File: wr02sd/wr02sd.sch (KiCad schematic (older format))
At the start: 9 parts

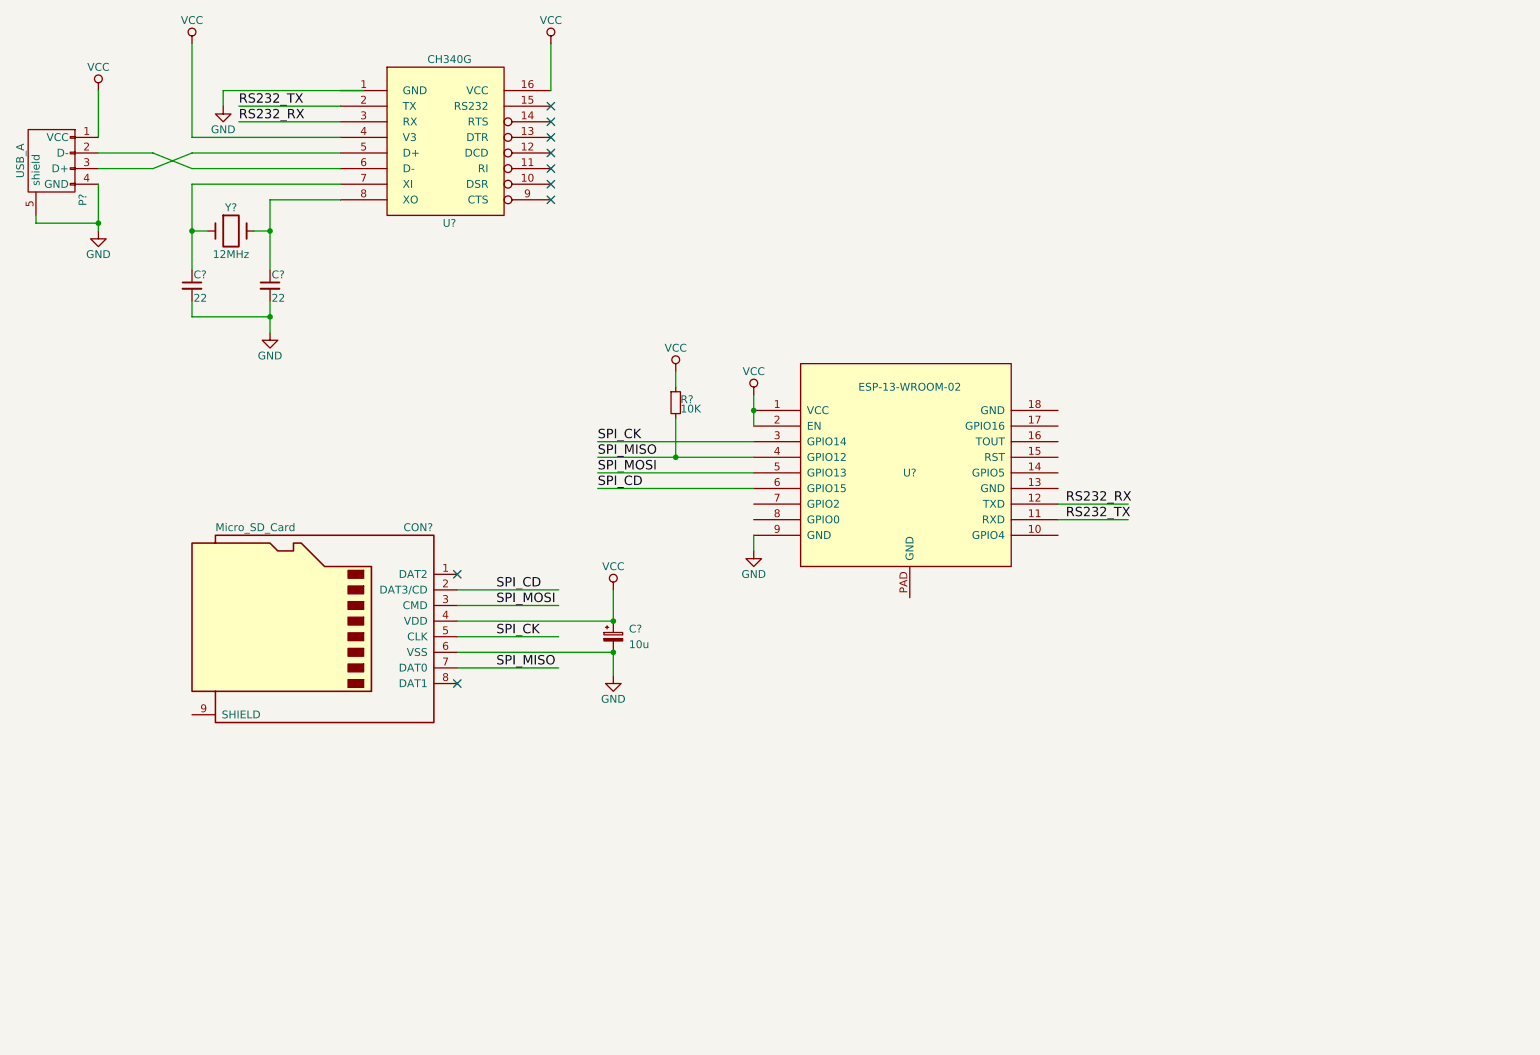
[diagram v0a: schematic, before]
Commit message: PCB Artworking is progressing.
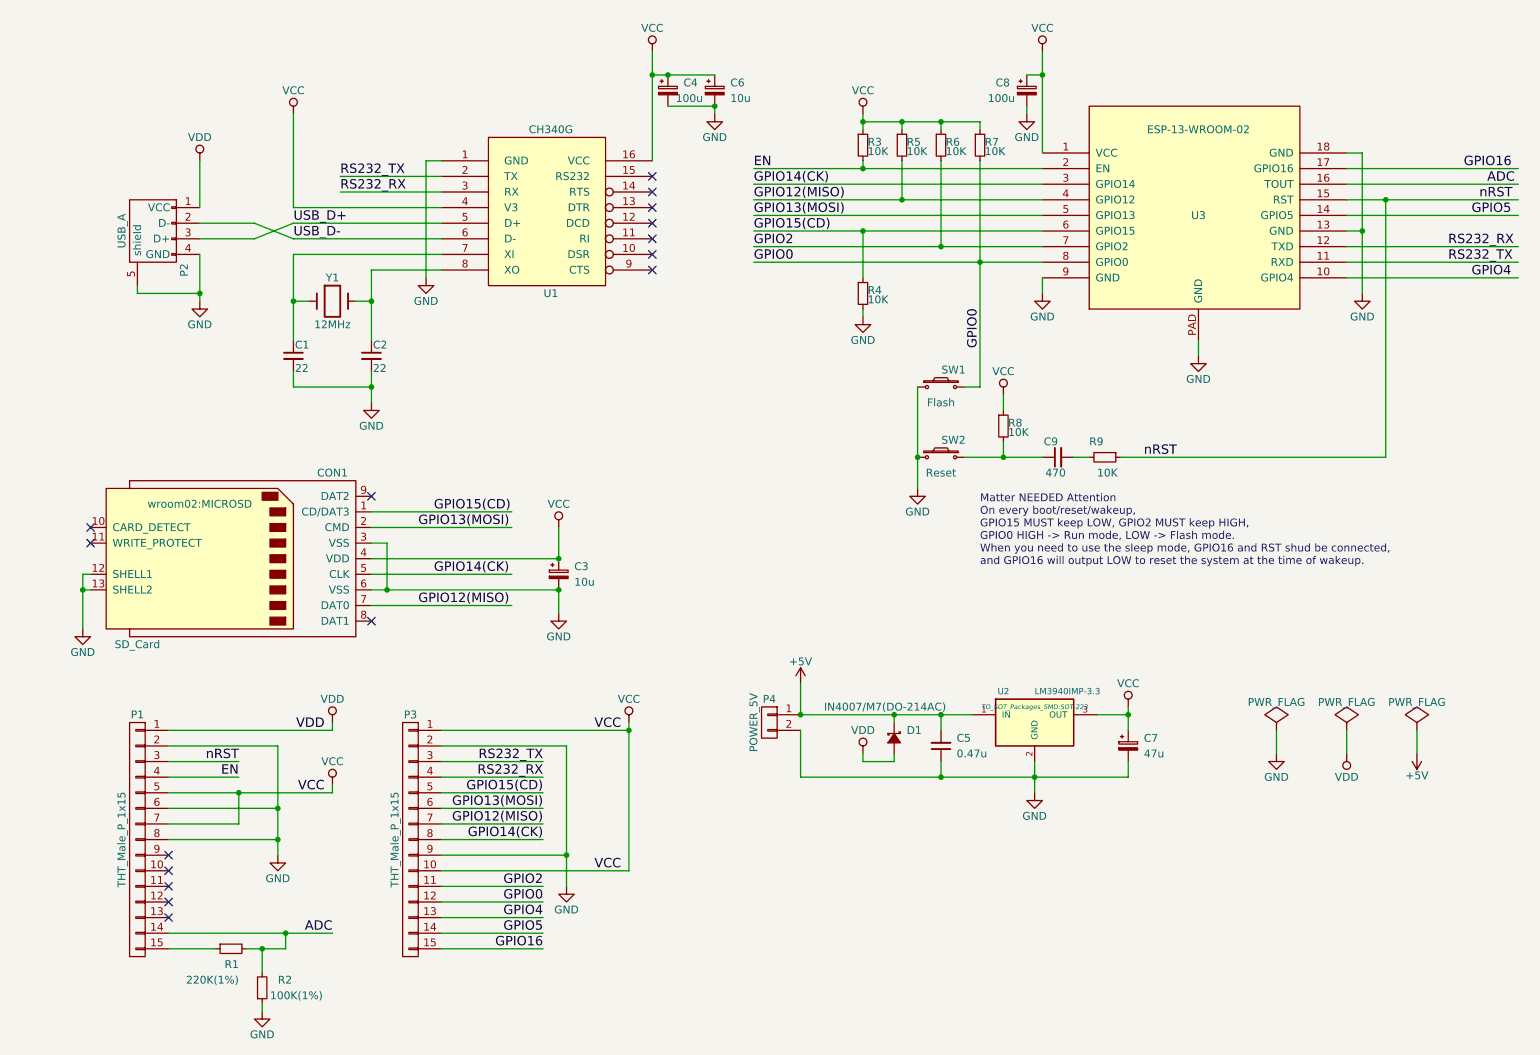
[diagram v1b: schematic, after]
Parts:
- removed CON?: Micro_SD_Card, symbol Micro_SD_Card
- added C4, C8: 100u, Capacitors_Tantalum_SMD:TantalC_SizeS_EIA-3216, symbol CP_Small
- added C5: 0.47u, Capacitors_SMD:C_1206, symbol C_Small
- added C6: 10u, Capacitors_SMD:C_1206, symbol CP_Small
- added C7: 47u, Capacitors_SMD:C_1210, symbol CP_Small
- added C9: 470, Capacitors_SMD:C_0805, symbol C_Small
- added CON1: SD_Card, wroom02:MICROSD, symbol SD_Card
- added D1: IN4007/M7(DO-214AC), Diodes_SMD:DO-214AB, symbol D_Schottky_Small
- added P1, P3: THT_Male_P_1x15, Pin_Headers:Pin_Header_Straight_1x15, symbol CONN_01X15
- added P4: POWER_5V, Connectors_JST:JST_PH_B2B-PH-K_02x2.00mm_Straight, symbol CONN_01X02
- added R1: 220K(1%), Resistors_SMD:R_0402, symbol R_Small
- added R2: 100K(1%), Resistors_SMD:R_0402, symbol R_Small
- added R4, R5, R6, R7, R8, R9: 10K, Resistors_SMD:R_0201, symbol R_Small
- added SW1: Flash, Buttons_Switches_SMD:SW_SPST_B3U-1000P, symbol SW_PUSH_SMALL_H
- added SW2: Reset, Buttons_Switches_SMD:SW_SPST_B3U-1000P, symbol SW_PUSH_SMALL_H
- added U2: LM3940IMP-3.3, TO_SOT_Packages_SMD:SOT-223, symbol LM3940IMP-3.3
- C1, C2: renamed from C?; footprint (none) -> Capacitors_SMD:C_0201
- C3: renamed from C?; footprint (none) -> Capacitors_SMD:C_1206
- P2: renamed from P?; footprint (none) -> Connect:USB_Micro-B
- R3: renamed from R?; footprint (none) -> Resistors_SMD:R_0201
- U1: renamed from U?; footprint (none) -> Housings_SOIC:SOIC-16_3.9x9.9mm_Pitch1.27mm
- U3: renamed from U?; footprint (none) -> wroom02:ESP-13-WROOM-02
- Y1: renamed from Y?; footprint (none) -> wroom02:smd_xtal
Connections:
- net labels added: +5V, ADC, EN, GPIO0, GPIO12(MISO), GPIO13(MOSI), GPIO14(CK), GPIO15(CD), GPIO16, GPIO2, GPIO4, GPIO5, USB_D+, USB_D-, VDD, nRST
- net labels removed: SPI_CD, SPI_CK, SPI_MISO, SPI_MOSI
- wire segments 45 -> 136
- no-connect marks 9 -> 16
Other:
- note added: "Matter NEEDED Attention\nOn every boot/reset/wakeup,\nGPIO15 MUST keep LOW, GPIO2 MUST keep HIGH,\nGPIO0 HIGH -> Run mode, LOW -> Flash mode.\nWhen you need to use the sleep mode, GPIO16 and RST shud be connected,\nand GPIO16 will output LOW to reset the system at the time of wakeup."
- moved on the sheet: C1, C2, C3, P2, R3, U1, U3, Y1

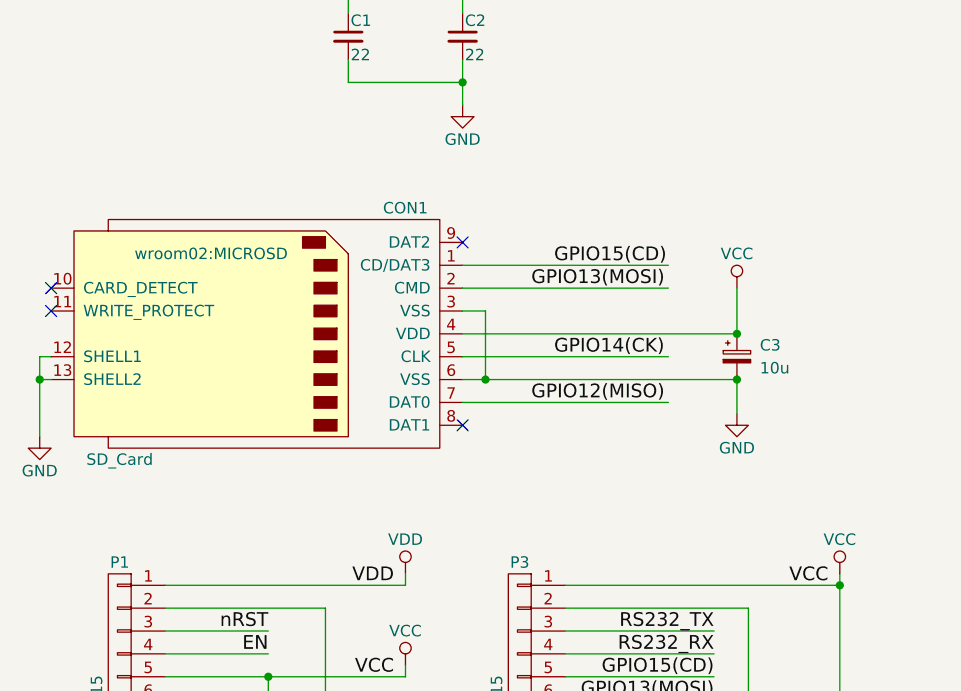
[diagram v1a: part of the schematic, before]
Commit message: PCB Artworking is progressing..
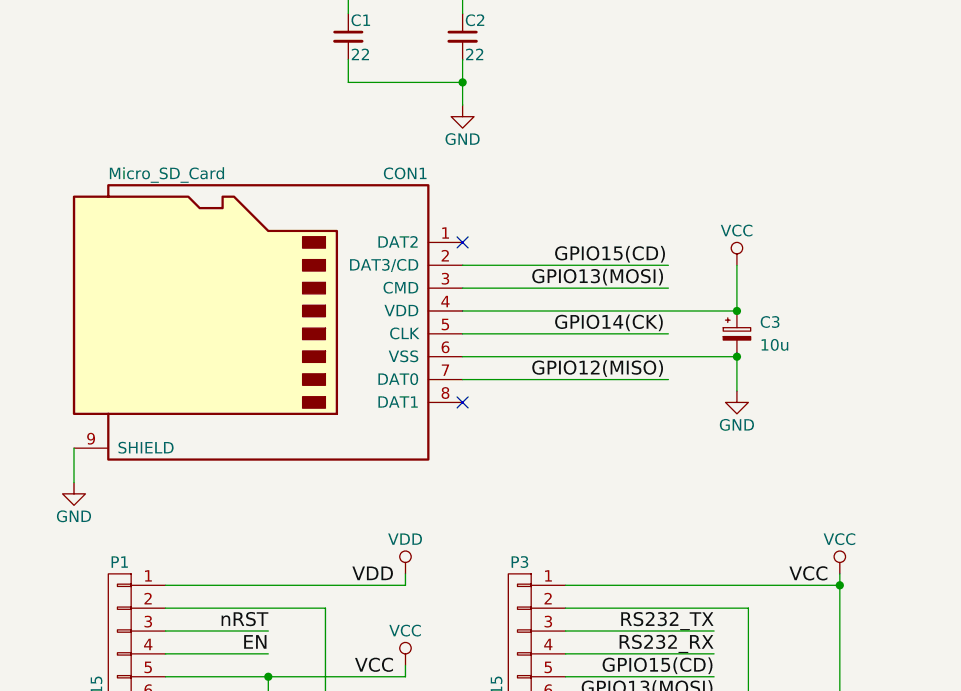
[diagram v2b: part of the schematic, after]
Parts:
- removed CON1: SD_Card, wroom02:MICROSD, symbol SD_Card
- added CON1: Micro_SD_Card, wroom02:MICROSD, symbol Micro_SD_Card
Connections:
- wire segments 136 -> 132
- no-connect marks 16 -> 14
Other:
- moved on the sheet: C3
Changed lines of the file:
@@
 	1    0    0    -1
 $EndComp
-NoConn ~ 3050 4800
-Text Label 3450 4500 0    60   ~ 0
+NoConn ~ 3050 4700
+Text Label 3450 4400 0    60   ~ 0
 GPIO14(CK)
-Text Label 3350 4700 0    60   ~ 0
+Text Label 3350 4600 0    60   ~ 0
 GPIO12(MISO)
 Text Label 3350 4200 0    60   ~ 0
@@
 L CP_Small C3
 U 1 1 57BD60BD
-P 4250 4500
-F 0 "C3" H 4350 4550 50  0000 L CNN
-F 1 "10u" H 4350 4450 50  0000 L CNN
-F 2 "Capacitors_SMD:C_1206" H 4250 4500 50  0001 C CNN
-F 3 "" H 4250 4500 50  0000 C CNN
-	1    4250 4500
+P 4250 4400
+F 0 "C3" H 4350 4450 50  0000 L CNN
+F 1 "10u" H 4350 4350 50  0000 L CNN
+F 2 "Capacitors_SMD:C_1206" H 4250 4400 50  0001 C CNN
+F 3 "" H 4250 4400 50  0000 C CNN
+	1    4250 4400
 	1    0    0    -1
 $EndComp
@@
 L GND #PWR06
 U 1 1 57BD62C3
-P 4250 4750
-F 0 "#PWR06" H 4250 4500 50  0001 C CNN
-F 1 "GND" H 4250 4600 50  0000 C CNN
-F 2 "" H 4250 4750 50  0000 C CNN
-F 3 "" H 4250 4750 50  0000 C CNN
-	1    4250 4750
+P 4250 4650
+F 0 "#PWR06" H 4250 4400 50  0001 C CNN
+F 1 "GND" H 4250 4500 50  0000 C CNN
+F 2 "" H 4250 4650 50  0000 C CNN
+F 3 "" H 4250 4650 50  0000 C CNN
+	1    4250 4650
 	1    0    0    -1
 $EndComp
@@
 L VCC #PWR07
 U 1 1 57BD62EE
-P 4250 4200
-F 0 "#PWR07" H 4250 4050 50  0001 C CNN
-F 1 "VCC" H 4250 4350 50  0000 C CNN
-F 2 "" H 4250 4200 50  0000 C CNN
-F 3 "" H 4250 4200 50  0000 C CNN
-	1    4250 4200
+P 4250 4100
+F 0 "#PWR07" H 4250 3950 50  0001 C CNN
+F 1 "VCC" H 4250 4250 50  0000 C CNN
+F 2 "" H 4250 4100 50  0000 C CNN
+F 3 "" H 4250 4100 50  0000 C CNN
+	1    4250 4100
 	1    0    0    -1
 $EndComp
@@
 	3050 3300 2550 3300
 Wire Wire Line
-	3050 4400 4250 4400
-Wire Wire Line
-	4250 4400 4250 4200
-Wire Wire Line
-	3050 4600 4250 4600
-Wire Wire Line
-	4250 4600 4250 4750
+	3050 4300 4250 4300
+Wire Wire Line
+	4250 4300 4250 4100
+Wire Wire Line
+	3050 4500 4250 4500
+Wire Wire Line
+	4250 4500 4250 4650
 Wire Wire Line
 	7350 2200 5500 2200
@@
 	5500 2100 7350 2100
 Wire Wire Line
-	3950 4700 3050 4700
+	3950 4600 3050 4600
 Wire Wire Line
 	5500 2300 7350 2300
@@
 	7350 2000 5500 2000
 Wire Wire Line
-	3950 4500 3050 4500
-Connection ~ 4250 4400
-Connection ~ 4250 4600
+	3950 4400 3050 4400
+Connection ~ 4250 4300
+Connection ~ 4250 4500
 Wire Wire Line
 	2550 3300 2550 3200
@@
 Connection ~ 4700 5500
 $Comp
-L SD_Card CON1
-U 1 1 57BE9D62
-P 2150 4400
-F 0 "CON1" H 1500 4950 50  0000 C CNN
-F 1 "SD_Card" H 2750 3850 50  0000 C CNN
-F 2 "wroom02:MICROSD" H 2350 4750 50  0000 C CNN
-F 3 "" H 2150 4400 50  0000 C CNN
-	1    2150 4400
-	-1   0    0    -1
-$EndComp
-NoConn ~ 3050 4000
-Wire Wire Line
-	3050 4300 3150 4300
-Wire Wire Line
-	3150 4300 3150 4600
-Connection ~ 3150 4600
-$Comp
 L GND #PWR035
 U 1 1 57BEA6E2
-P 1200 4850
-F 0 "#PWR035" H 1200 4600 50  0001 C CNN
-F 1 "GND" H 1200 4700 50  0000 C CNN
-F 2 "" H 1200 4850 50  0000 C CNN
-F 3 "" H 1200 4850 50  0000 C CNN
-	1    1200 4850
-	1    0    0    -1
-$EndComp
-Wire Wire Line
-	1200 4500 1200 4850
-Wire Wire Line
-	1250 4500 1200 4500
-Wire Wire Line
-	1250 4600 1200 4600
-Connection ~ 1200 4600
-NoConn ~ 1250 4200
-NoConn ~ 1250 4300
+P 1350 5050
+F 0 "#PWR035" H 1350 4800 50  0001 C CNN
+F 1 "GND" H 1350 4900 50  0000 C CNN
+F 2 "" H 1350 5050 50  0000 C CNN
+F 3 "" H 1350 5050 50  0000 C CNN
+	1    1350 5050
+	1    0    0    -1
+$EndComp
+NoConn ~ 3050 4000
+$Comp
+L Micro_SD_Card CON1
+U 1 1 57BF871D
+P 2150 4300
+F 0 "CON1" H 1500 4900 50  0000 C CNN
+F 1 "Micro_SD_Card" H 2800 4900 50  0000 R CNN
+F 2 "wroom02:MICROSD" H 3300 4600 50  0001 C CNN
+F 3 "" H 2150 4300 50  0000 C CNN
+	1    2150 4300
+	-1   0    0    -1
+$EndComp
+Wire Wire Line
+	1350 4900 1350 5050
 $EndSCHEMATC
